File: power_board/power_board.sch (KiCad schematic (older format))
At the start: 67 parts, among them J1 PROG, J10 M4, J11 5V_1, J12 M5, J13 M6, J14 M7, J15 FAN, J16 Screw_Terminal_01x02, J17 MB_interface, J18 Conn_01x02_Female, J19 12V_1, J2 M1, J20 12V_2, J21 12V_3, J22 12V_4, J23 48V_1, J24 48V_2, J25 48V_3, J26 48V_4, J3 M2, J4 Conn_01x02_Female, J5 Conn_01x02_Female, J6 Conn_01x01_Male, J7 Conn_01x01_Male, J8 Screw_Terminal_01x02, J9 M3, Q1 2N3906, SW1 SW_Push, U1 ACS758xCB-050B-PFF, U2 ACS758xCB-050B-PFF, U3 MCP2515-EST, U4 MAX31855KASA, U5 MCP2551-I-SN, U6 BTS50085-1TMA, U7 ATmega328P-AU, U8 BTS50085-1TMA, U9 LM2596S-5, Y1 20Mhz, Y2 16Mhz

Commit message: working on microcontroller routing
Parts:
- D2, D3: footprint Diode_SMD:D_0603_1608Metric -> Diode_SMD:D_SMB
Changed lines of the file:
@@
 F 0 "D2" H 7000 2000 50  0000 C CNN
 F 1 "1N5824" H 7000 2200 50  0000 C CNN
-F 2 "Diode_SMD:D_0603_1608Metric" H 7000 2100 50  0001 C CNN
+F 2 "Diode_SMD:D_SMB" H 7000 2100 50  0001 C CNN
 F 3 "~" H 7000 2100 50  0001 C CNN
 	1    7000 2100
@@
 F 0 "D3" H 7800 1684 50  0000 C CNN
 F 1 "--" H 7800 1775 50  0000 C CNN
-F 2 "Diode_SMD:D_0603_1608Metric" H 7800 1900 50  0001 C CNN
+F 2 "Diode_SMD:D_SMB" H 7800 1900 50  0001 C CNN
 F 3 "~" H 7800 1900 50  0001 C CNN
 	1    7800 1900

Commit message: finishing touches
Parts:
- Y2: footprint Crystal:Resonator_SMD-3Pin_7.2x3.0mm -> CSTCE16M0V53-R0:OSC_CSTCE16M0V53-R0
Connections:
- wire segments 284 -> 288
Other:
- note added: "D4"
- moved on the sheet: C1, C2
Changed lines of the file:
@@
 L Device:CP C1
 U 1 1 5BA44640
-P 2600 4650
-F 0 "C1" H 2500 4450 50  0000 L CNN
-F 1 "300uF" H 2500 4350 50  0000 L CNN
-F 2 "Capacitor_THT:CP_Radial_D10.0mm_P7.50mm" H 2638 4500 50  0001 C CNN
-F 3 "~" H 2600 4650 50  0001 C CNN
-	1    2600 4650
+P 1350 3850
+F 0 "C1" H 1150 3950 50  0000 L CNN
+F 1 "300uF" H 1100 3750 50  0000 L CNN
+F 2 "Capacitor_THT:CP_Radial_D10.0mm_P7.50mm" H 1388 3700 50  0001 C CNN
+F 3 "~" H 1350 3850 50  0001 C CNN
+	1    1350 3850
 	1    0    0    -1
 $EndComp
@@
 L Device:CP C2
 U 1 1 5BA446DC
-P 2600 5900
-F 0 "C2" H 2500 5700 50  0000 L CNN
-F 1 "300uF" H 2500 5600 50  0000 L CNN
-F 2 "Capacitor_THT:CP_Radial_D10.0mm_P7.50mm" H 2638 5750 50  0001 C CNN
-F 3 "~" H 2600 5900 50  0001 C CNN
-	1    2600 5900
+P 1650 3850
+F 0 "C2" H 1700 3950 50  0000 L CNN
+F 1 "300uF" H 1100 3750 50  0000 L CNN
+F 2 "Capacitor_THT:CP_Radial_D10.0mm_P7.50mm" H 1688 3700 50  0001 C CNN
+F 3 "~" H 1650 3850 50  0001 C CNN
+	1    1650 3850
 	1    0    0    -1
 $EndComp
@@
 	12800 7800 12800 7700
 $Comp
-L Device:Resonator Y2
-U 1 1 5BA74C01
-P 15050 5650
-F 0 "Y2" V 15350 5500 50  0000 L CNN
-F 1 "16Mhz" V 15250 5350 50  0000 L CNN
-F 2 "Crystal:Resonator_SMD-3Pin_7.2x3.0mm" H 15025 5650 50  0001 C CNN
-F 3 "~" H 15025 5650 50  0001 C CNN
-	1    15050 5650
-	0    -1   -1   0
-$EndComp
-$Comp
 L power:GNDREF #PWR0125
 U 1 1 5BA7A004
@@
 	1    0    0    -1
 $EndComp
+Text GLabel 14650 6000 2    50   Input ~ 0
+12V_SENSE
 Text GLabel 14650 5900 2    50   Input ~ 0
-12V_SENSE
-Text GLabel 14650 6000 2    50   Input ~ 0
 12VA_SENSE
 Wire Wire Line
@@
 Text GLabel 14800 5350 2    50   Input ~ 0
 SCK
-Text GLabel 14600 7300 2    50   Input ~ 0
+Text GLabel 14600 7100 2    50   Input ~ 0
 TC_CS
 Wire Wire Line
-	14500 7300 14600 7300
-Wire Wire Line
 	14800 5600 14800 5500
 Wire Wire Line
@@
 	14800 5700 14800 5800
 Wire Wire Line
-	14800 5800 15050 5800
-Wire Wire Line
 	14500 5700 14800 5700
-Wire Wire Line
-	15250 5650 15400 5650
 $Comp
 L Device:R_US R8
@@
 Wire Wire Line
 	8200 8550 8250 8550
-Text GLabel 14600 6900 2    50   Input ~ 0
+Text GLabel 14600 7000 2    50   Input ~ 0
 CAN_INT
 Wire Wire Line
@@
 	1    0    0    -1
 $EndComp
+Text GLabel 9250 5550 0    50   Input ~ 0
+TX
 Text GLabel 9250 5450 0    50   Input ~ 0
-TX
-Text GLabel 9250 5550 0    50   Input ~ 0
 RX
 Wire Wire Line
@@
 L power:GNDREF #PWR0101
 U 1 1 5BABAFE5
-P 2850 4950
-F 0 "#PWR0101" H 2850 4700 50  0001 C CNN
-F 1 "GNDREF" H 2855 4777 50  0000 C CNN
-F 2 "" H 2850 4950 50  0001 C CNN
-F 3 "" H 2850 4950 50  0001 C CNN
-	1    2850 4950
+P 1500 4000
+F 0 "#PWR0101" H 1500 3750 50  0001 C CNN
+F 1 "GNDREF" H 1505 3827 50  0000 C CNN
+F 2 "" H 1500 4000 50  0001 C CNN
+F 3 "" H 1500 4000 50  0001 C CNN
+	1    1500 4000
 	1    0    0    -1
 $EndComp
@@
 Wire Wire Line
 	8200 8650 8250 8650
-Text GLabel 14600 7000 2    50   Input ~ 0
+Text GLabel 14600 6900 2    50   Input ~ 0
 RX_INT
 Wire Wire Line
@@
 Text GLabel 14650 6100 2    50   Input ~ 0
 RX1BF
-Text GLabel 14650 6200 2    50   Input ~ 0
+Text GLabel 14650 6400 2    50   Input ~ 0
 TX0RTS
 Text GLabel 14650 6300 2    50   Input ~ 0
 TX1RTS
-Text GLabel 14650 6400 2    50   Input ~ 0
+Text GLabel 14650 6200 2    50   Input ~ 0
 TX2RTS
 Wire Wire Line
@@
 	2850 4650 2850 4800
 Connection ~ 2850 4800
-Connection ~ 2600 4500
-Wire Wire Line
-	2600 4500 2450 4500
-Wire Wire Line
-	2600 4500 2900 4500
-Wire Wire Line
-	2600 4800 2850 4800
 Connection ~ 2600 5750
 Wire Wire Line
 	2600 5750 2450 5750
-Wire Wire Line
-	2850 6050 2600 6050
 Wire Wire Line
 	2600 5750 2900 5750
@@
 NoConn ~ 9350 8300
 NoConn ~ 14500 7400
-NoConn ~ 14500 7100
+NoConn ~ 14500 7300
 NoConn ~ 14500 5000
 NoConn ~ 14500 5100
@@
 L power:+5V #PWR0159
 U 1 1 5BC39A5C
-P 11350 5400
-F 0 "#PWR0159" H 11350 5250 50  0001 C CNN
-F 1 "+5V" H 11365 5573 50  0000 C CNN
-F 2 "" H 11350 5400 50  0001 C CNN
-F 3 "" H 11350 5400 50  0001 C CNN
-	1    11350 5400
+P 11200 5950
+F 0 "#PWR0159" H 11200 5800 50  0001 C CNN
+F 1 "+5V" H 11215 6123 50  0000 C CNN
+F 2 "" H 11200 5950 50  0001 C CNN
+F 3 "" H 11200 5950 50  0001 C CNN
+	1    11200 5950
 	1    0    0    -1
 $EndComp
@@
 L power:GNDREF #PWR0160
 U 1 1 5BC39AEB
-P 11350 5800
-F 0 "#PWR0160" H 11350 5550 50  0001 C CNN
-F 1 "GNDREF" H 11355 5627 50  0000 C CNN
-F 2 "" H 11350 5800 50  0001 C CNN
-F 3 "" H 11350 5800 50  0001 C CNN
-	1    11350 5800
-	1    0    0    -1
-$EndComp
-Wire Wire Line
-	11350 5450 11350 5400
-Wire Wire Line
-	11350 5800 11350 5750
+P 11750 5300
+F 0 "#PWR0160" H 11750 5050 50  0001 C CNN
+F 1 "GNDREF" H 11755 5127 50  0000 C CNN
+F 2 "" H 11750 5300 50  0001 C CNN
+F 3 "" H 11750 5300 50  0001 C CNN
+	1    11750 5300
+	1    0    0    -1
+$EndComp
 Text GLabel 11250 5550 0    50   Input ~ 0
 CANH
@@
 Wire Wire Line
 	1400 8400 1400 8650
+Wire Wire Line
+	14800 5800 15050 5800
+Wire Wire Line
+	15250 5650 15400 5650
+$Comp
+L Device:Resonator Y2
+U 1 1 5BA74C01
+P 15050 5650
+F 0 "Y2" V 15350 5500 50  0000 L CNN
+F 1 "16Mhz" V 15250 5350 50  0000 L CNN
+F 2 "CSTCE16M0V53-R0:OSC_CSTCE16M0V53-R0" H 15025 5650 50  0001 C CNN
+F 3 "~" H 15025 5650 50  0001 C CNN
+	1    15050 5650
+	0    -1   -1   0
+$EndComp
+Wire Wire Line
+	14500 7100 14600 7100
+Text Notes 14200 7150 2    50   ~ 0
+D4
+Wire Wire Line
+	11200 5950 11350 5950
+Wire Wire Line
+	11350 5950 11350 5750
+Wire Wire Line
+	11350 5450 11350 5300
+Wire Wire Line
+	11350 5300 11750 5300
+Wire Wire Line
+	2450 4500 2900 4500
+Wire Wire Line
+	1650 4000 1500 4000
+Wire Wire Line
+	1350 4000 1500 4000
+Connection ~ 1500 4000
+Wire Wire Line
+	1650 3700 1500 3700
+$Comp
+L power:+48V #PWR0161
+U 1 1 5BD4F164
+P 1500 3650
+F 0 "#PWR0161" H 1500 3500 50  0001 C CNN
+F 1 "+48V" H 1515 3823 50  0000 C CNN
+F 2 "" H 1500 3650 50  0001 C CNN
+F 3 "" H 1500 3650 50  0001 C CNN
+	1    1500 3650
+	1    0    0    -1
+$EndComp
+Wire Wire Line
+	1500 3650 1500 3700
+Connection ~ 1500 3700
+Wire Wire Line
+	1500 3700 1350 3700
+$Comp
+L power:GNDREF #PWR?
+U 1 1 5BD67F28
+P 2850 4950
+F 0 "#PWR?" H 2850 4700 50  0001 C CNN
+F 1 "GNDREF" H 2855 4777 50  0000 C CNN
+F 2 "" H 2850 4950 50  0001 C CNN
+F 3 "" H 2850 4950 50  0001 C CNN
+	1    2850 4950
+	1    0    0    -1
+$EndComp
 $EndSCHEMATC

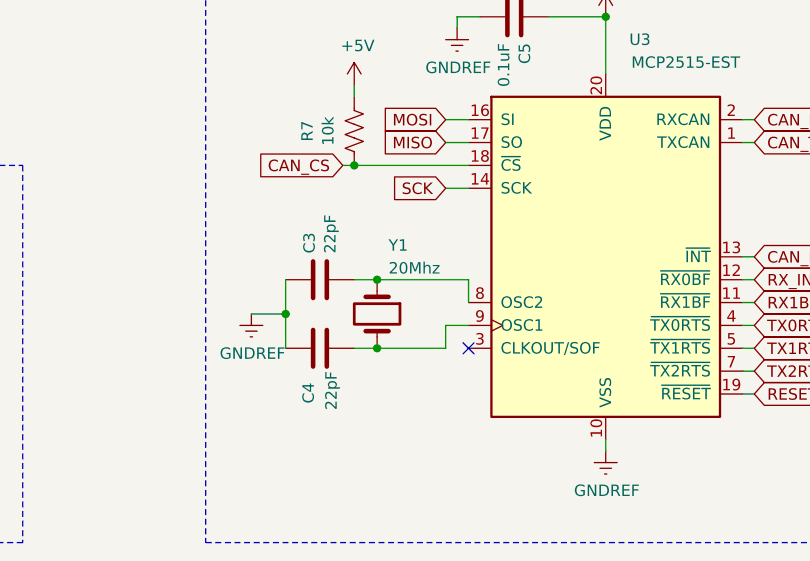
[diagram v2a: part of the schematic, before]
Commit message: Finished final Draft of design
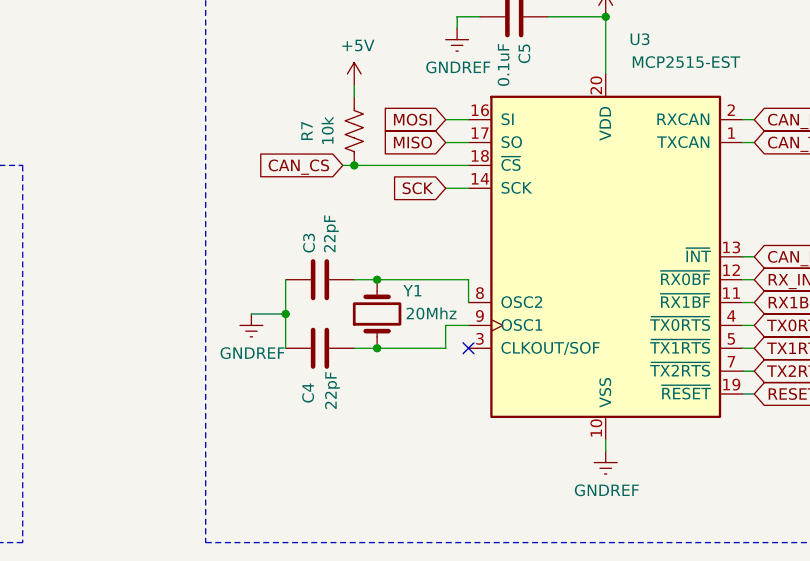
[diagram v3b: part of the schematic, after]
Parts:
- Y1: footprint Crystal:Resonator_SMD-3Pin_7.2x3.0mm -> Crystal:Crystal_SMD_0603-2Pin_6.0x3.5mm
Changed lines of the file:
@@
 U 1 1 5BB39D19
 P 6600 8800
-F 0 "Y1" V 6300 8850 50  0000 L CNN
-F 1 "20Mhz" V 6400 8850 50  0000 L CNN
-F 2 "Crystal:Resonator_SMD-3Pin_7.2x3.0mm" H 6600 8800 50  0001 C CNN
+F 0 "Y1" V 6700 8600 50  0000 L CNN
+F 1 "20Mhz" V 6600 8450 50  0000 L CNN
+F 2 "Crystal:Crystal_SMD_0603-2Pin_6.0x3.5mm" H 6600 8800 50  0001 C CNN
 F 3 "~" H 6600 8800 50  0001 C CNN
 	1    6600 8800
-	0    1    1    0
+	0    -1   -1   0
 $EndComp
 $Comp
@@
 	1500 3700 1350 3700
 $Comp
-L power:GNDREF #PWR?
+L power:GNDREF #PWR0162
 U 1 1 5BD67F28
 P 2850 4950
-F 0 "#PWR?" H 2850 4700 50  0001 C CNN
+F 0 "#PWR0162" H 2850 4700 50  0001 C CNN
 F 1 "GNDREF" H 2855 4777 50  0000 C CNN
 F 2 "" H 2850 4950 50  0001 C CNN
